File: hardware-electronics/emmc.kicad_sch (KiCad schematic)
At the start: 44 parts, among them U2 EMMC16G-MW28-01E10, U4 24AA04T-I_OT, U8 USB2244-AEZG-06, Y2 ECS-240-10-47-CKM-TR

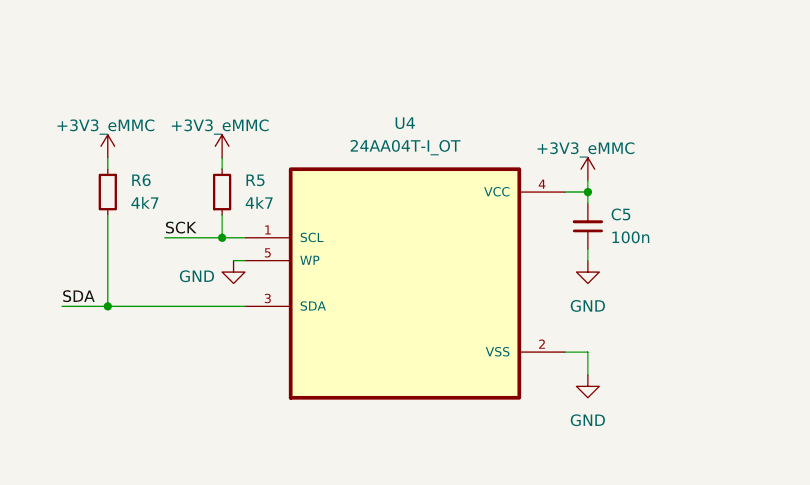
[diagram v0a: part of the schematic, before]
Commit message: SCH update all symbols
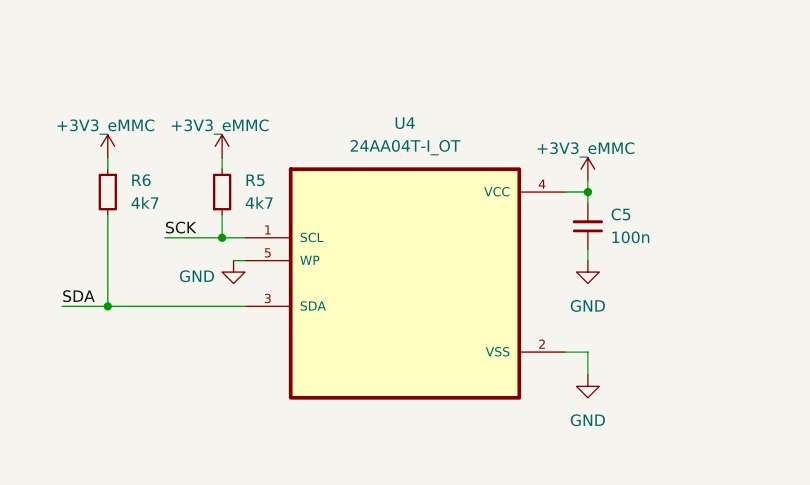
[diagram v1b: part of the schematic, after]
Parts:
- C10, C4: footprint C_4pF_0402:C_0402_1005Metric -> M2SmartHomeFootprints:C_0402
- C11, C12, C14, C17, C21, C7, C9: footprint C_1uF_0402:C_0402_1005Metric -> M2SmartHomeFootprints:C_0201
- C13, C15, C16, C19, C22, C3, C5, C6, C8: footprint C_100n_0402:C_0402_1005Metric -> M2SmartHomeFootprints:C_0402
- C18, C23: footprint C_4u7_0402:C_0402_1005Metric -> M2SmartHomeFootprints:C_0402
- FB1: footprint FB_120R_0603:FB_0603_1608Metric -> M2SmartHomeFootprints:FB_0603
- R10, R4: footprint R_0_0402:R_0402_1005Metric -> M2SmartHomeFootprints:R_0402
- R11, R12, R13, R14, R15, R16, R17, R18, R20: footprint R_49k9_0402:R_0402_1005Metric -> M2SmartHomeFootprints:R_0402
- R19, R2: footprint R_10k_0402:R_0402_1005Metric -> M2SmartHomeFootprints:R_0402
- R5, R6: footprint R_4k7_0402:R_0402_1005Metric -> M2SmartHomeFootprints:R_0402
- R7: footprint R_12k_0402:R_0402_1005Metric -> M2SmartHomeFootprints:R_0402
- R8: footprint R_1M_0402:R_0402_1005Metric -> M2SmartHomeFootprints:R_0402
- R9: footprint R_500R_0402:R_0402_1005Metric -> M2SmartHomeFootprints:R_0402
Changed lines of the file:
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@@
 			)
 		)
-		(property "Footprint" "R_49k9_0402:R_0402_1005Metric"
+		(property "Footprint" "M2SmartHomeFootprints:R_0402"
 			(at 140.97 53.34 0)
 			(effects
@@
 			)
 		)
-		(property "Footprint" "C_100n_0402:C_0402_1005Metric"
+		(property "Footprint" "M2SmartHomeFootprints:C_0402"
 			(at 280.67 73.66 0)
 			(effects
@@
 			)
 		)
-		(property "Footprint" "R_0_0402:R_0402_1005Metric"
+		(property "Footprint" "M2SmartHomeFootprints:R_0402"
 			(at 142.24 91.44 0)
 			(effects
@@
 			)
 		)
-		(property "Footprint" "C_1uF_0402:C_0402_1005Metric"
+		(property "Footprint" "M2SmartHomeFootprints:C_0201"
 			(at 232.41 83.82 0)
 			(effects
@@
 			)
 		)
-		(property "Footprint" "C_4pF_0402:C_0402_1005Metric"
+		(property "Footprint" "M2SmartHomeFootprints:C_0402"
 			(at 63.5 137.16 0)
 			(effects
@@
 			)
 		)
-		(property "Footprint" "R_49k9_0402:R_0402_1005Metric"
+		(property "Footprint" "M2SmartHomeFootprints:R_0402"
 			(at 110.49 53.34 0)
 			(effects
@@
 			)
 		)
-		(property "Footprint" "R_10k_0402:R_0402_1005Metric"
+		(property "Footprint" "M2SmartHomeFootprints:R_0402"
 			(at 149.86 53.34 0)
 			(effects
@@
 			)
 		)
-		(property "Footprint" "R_49k9_0402:R_0402_1005Metric"
+		(property "Footprint" "M2SmartHomeFootprints:R_0402"
 			(at 105.41 53.34 0)
 			(effects
@@
 			)
 		)
-		(property "Footprint" "R_49k9_0402:R_0402_1005Metric"
+		(property "Footprint" "M2SmartHomeFootprints:R_0402"
 			(at 120.65 53.34 0)
 			(effects
@@
 			)
 		)
-		(property "Datasheet" ""
+		(property "Datasheet" "https://ww1.microchip.com/downloads/aemDocuments/documents/MPD/ProductDocuments/DataSheets/24AA04-24LC04B-24FC04-4K-I2C-Serial-EEPROM-20001708P.pdf"
 			(at 139.7 166.37 0)
 			(effects
@@
 			)
 		)
-		(property "Footprint" "C_1uF_0402:C_0402_1005Metric"
+		(property "Footprint" "M2SmartHomeFootprints:C_0201"
 			(at 215.9 91.44 0)
 			(effects
@@
 			)
 		)
-		(property "Footprint" "C_4u7_0402:C_0402_1005Metric"
+		(property "Footprint" "M2SmartHomeFootprints:C_0402"
 			(at 54.61 36.83 0)
 			(effects
@@
 			)
 		)
-		(property "Footprint" "C_4u7_0402:C_0402_1005Metric"
+		(property "Footprint" "M2SmartHomeFootprints:C_0402"
 			(at 96.52 36.83 0)
 			(effects
@@
 			)
 		)
-		(property "Footprint" "R_49k9_0402:R_0402_1005Metric"
+		(property "Footprint" "M2SmartHomeFootprints:R_0402"
 			(at 115.57 53.34 0)
 			(effects
@@
 			)
 		)
-		(property "Footprint" "C_100n_0402:C_0402_1005Metric"
+		(property "Footprint" "M2SmartHomeFootprints:C_0402"
 			(at 87.63 36.83 0)
 			(effects
@@
 			)
 		)
-		(property "Footprint" "C_100n_0402:C_0402_1005Metric"
+		(property "Footprint" "M2SmartHomeFootprints:C_0402"
 			(at 45.72 36.83 0)
 			(effects
@@
 			)
 		)
-		(property "Footprint" "C_100n_0402:C_0402_1005Metric"
+		(property "Footprint" "M2SmartHomeFootprints:C_0402"
 			(at 172.72 142.24 0)
 			(effects
@@
 			)
 		)
-		(property "Footprint" "C_100n_0402:C_0402_1005Metric"
+		(property "Footprint" "M2SmartHomeFootprints:C_0402"
 			(at 223.52 83.82 0)
 			(effects
@@
 			)
 		)
-		(property "Footprint" "C_4pF_0402:C_0402_1005Metric"
+		(property "Footprint" "M2SmartHomeFootprints:C_0402"
 			(at 46.99 137.16 0)
 			(effects
@@
 			)
 		)
-		(property "Footprint" "R_49k9_0402:R_0402_1005Metric"
+		(property "Footprint" "M2SmartHomeFootprints:R_0402"
 			(at 130.81 53.34 0)
 			(effects
@@
 			)
 		)
-		(property "Footprint" "R_4k7_0402:R_0402_1005Metric"
+		(property "Footprint" "M2SmartHomeFootprints:R_0402"
 			(at 134.62 138.43 0)
 			(effects
@@
 			)
 		)
-		(property "Footprint" "R_49k9_0402:R_0402_1005Metric"
+		(property "Footprint" "M2SmartHomeFootprints:R_0402"
 			(at 125.73 53.34 0)
 			(effects
@@
 			)
 		)
-		(property "Footprint" "R_49k9_0402:R_0402_1005Metric"
+		(property "Footprint" "M2SmartHomeFootprints:R_0402"
 			(at 146.05 53.34 0)
 			(effects
@@
 			)
 		)
-		(property "Footprint" "C_100n_0402:C_0402_1005Metric"
+		(property "Footprint" "M2SmartHomeFootprints:C_0402"
 			(at 207.01 91.44 0)
 			(effects
@@
 			)
 		)
-		(property "Footprint" "R_500R_0402:R_0402_1005Metric"
+		(property "Footprint" "M2SmartHomeFootprints:R_0402"
 			(at 184.15 64.77 0)
 			(effects
@@
 			)
 		)
-		(property "Footprint" "R_12k_0402:R_0402_1005Metric"
+		(property "Footprint" "M2SmartHomeFootprints:R_0402"
 			(at 203.2 95.25 0)
 			(effects
@@
 			)
 		)
-		(property "Footprint" "C_100n_0402:C_0402_1005Metric"
+		(property "Footprint" "M2SmartHomeFootprints:C_0402"
 			(at 38.1 66.04 0)
 			(effects
@@
 			)
 		)
-		(property "Footprint" "R_0_0402:R_0402_1005Metric"
+		(property "Footprint" "M2SmartHomeFootprints:R_0402"
 			(at 151.13 91.44 0)
 			(effects
@@
 			)
 		)
-		(property "Footprint" "FB_120R_0603:FB_0603_1608Metric"
+		(property "Footprint" "M2SmartHomeFootprints:FB_0603"
 			(at 260.35 106.68 0)
 			(effects
@@
 			)
 		)
-		(property "Footprint" "C_1uF_0402:C_0402_1005Metric"
+		(property "Footprint" "M2SmartHomeFootprints:C_0201"
 			(at 273.05 80.01 0)
 			(effects
@@
 			)
 		)
-		(property "Footprint" "C_100n_0402:C_0402_1005Metric"
+		(property "Footprint" "M2SmartHomeFootprints:C_0402"
 			(at 241.3 83.82 0)
 			(effects
@@
 			)
 		)
-		(property "Footprint" "R_4k7_0402:R_0402_1005Metric"
+		(property "Footprint" "M2SmartHomeFootprints:R_0402"
 			(at 91.44 173.99 0)
 			(effects
@@
 			)
 		)
-		(property "Footprint" "C_1uF_0402:C_0402_1005Metric"
+		(property "Footprint" "M2SmartHomeFootprints:C_0201"
 			(at 29.21 66.04 0)
 			(effects
@@
 			)
 		)
-		(property "Footprint" "C_100n_0402:C_0402_1005Metric"
+		(property "Footprint" "M2SmartHomeFootprints:C_0402"
 			(at 264.16 80.01 0)
 			(effects
@@
 			)
 		)
-		(property "Footprint" "C_1uF_0402:C_0402_1005Metric"
+		(property "Footprint" "M2SmartHomeFootprints:C_0201"
 			(at 250.19 83.82 0)
 			(effects
@@
 			)
 		)
-		(property "Footprint" "R_49k9_0402:R_0402_1005Metric"
+		(property "Footprint" "M2SmartHomeFootprints:R_0402"
 			(at 135.89 53.34 0)
 			(effects
@@
 			)
 		)
-		(property "Footprint" "R_1M_0402:R_0402_1005Metric"
+		(property "Footprint" "M2SmartHomeFootprints:R_0402"
 			(at 60.96 163.83 0)
 			(effects
@@
 			)
 		)
-		(property "Footprint" "C_1uF_0402:C_0402_1005Metric"
+		(property "Footprint" "M2SmartHomeFootprints:C_0201"
 			(at 90.17 156.21 0)
 			(effects
@@
 			)
 		)
-		(property "Footprint" "C_1uF_0402:C_0402_1005Metric"
+		(property "Footprint" "M2SmartHomeFootprints:C_0201"
 			(at 289.56 73.66 0)
 			(effects
@@
 			)
 		)
-		(property "Footprint" "R_10k_0402:R_0402_1005Metric"
+		(property "Footprint" "M2SmartHomeFootprints:R_0402"
 			(at 92.71 143.51 0)
 			(effects
